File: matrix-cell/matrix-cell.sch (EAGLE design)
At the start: 4 parts

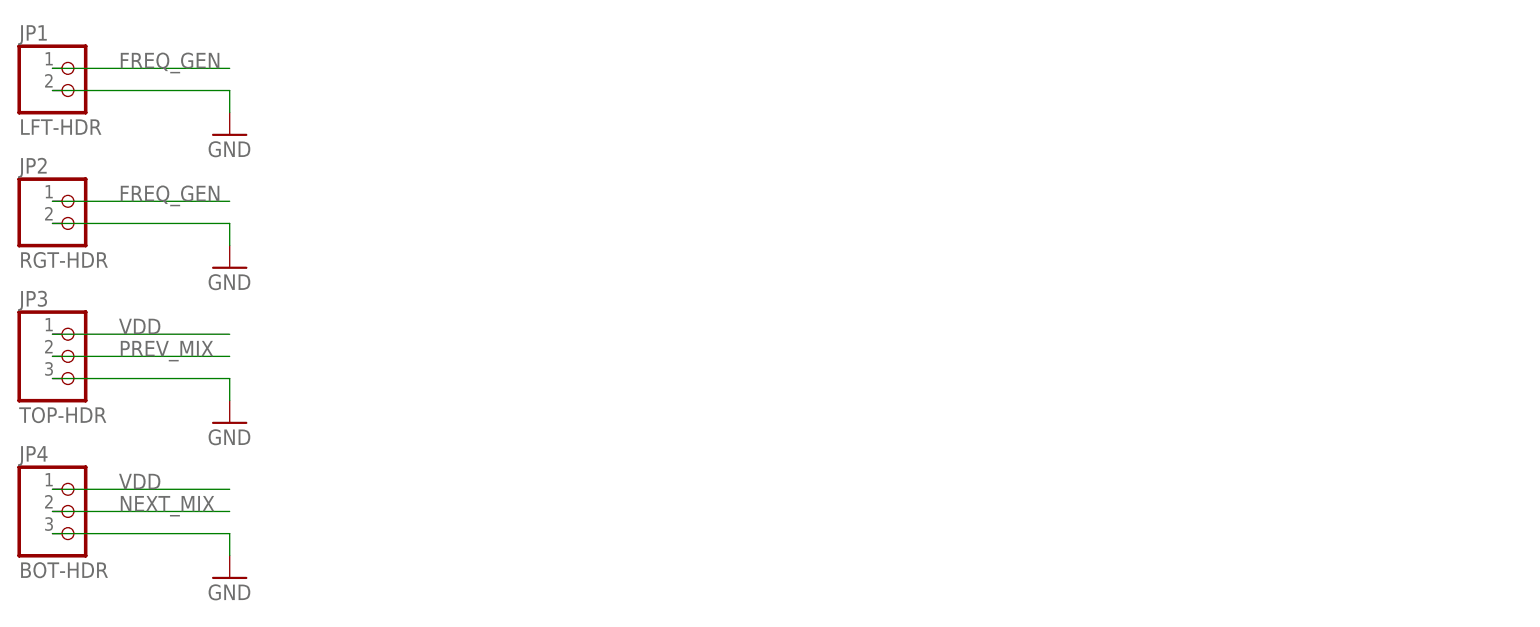
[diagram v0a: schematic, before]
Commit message: finished cell
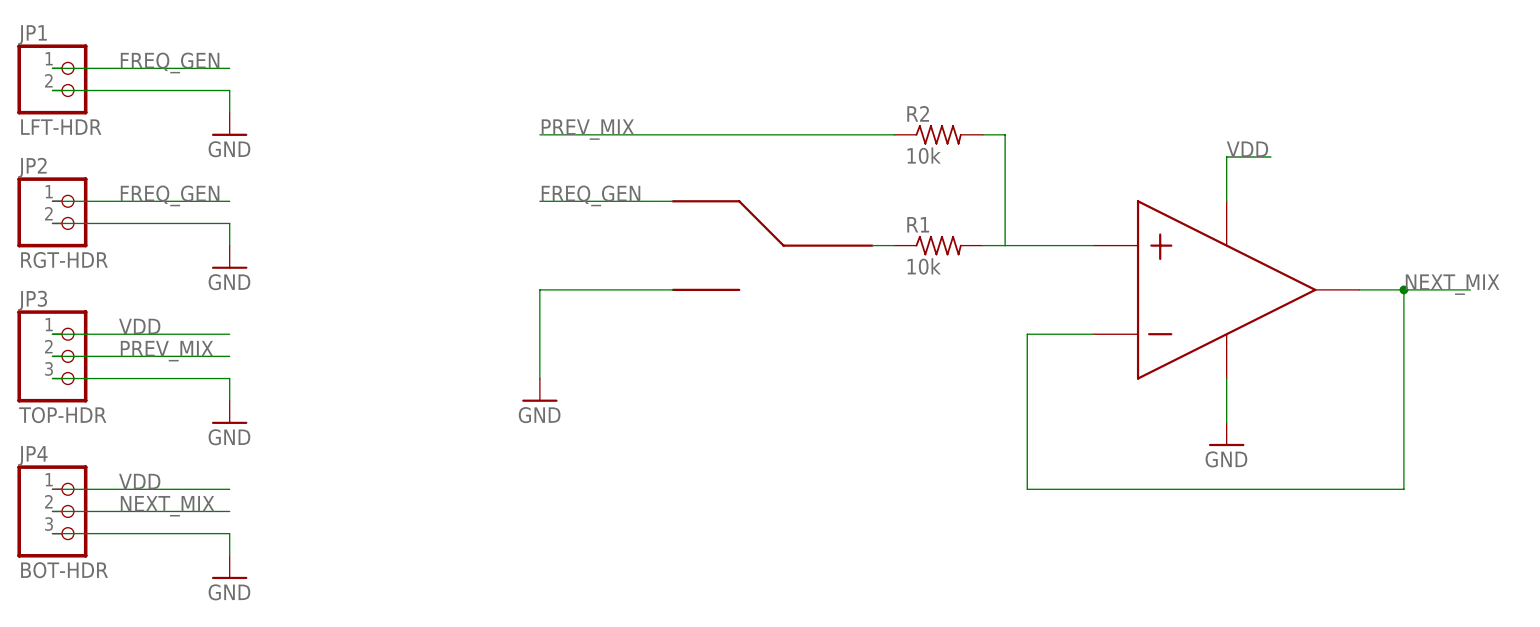
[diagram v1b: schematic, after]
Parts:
- added R1, R2: 10k, rcl:R-US_R1206
- added U$1: RA1-SWITCH, Tone-Matrix:RA1-SWITCH
- added U$2: MCP4162-OPAMP, Tone-Matrix:MCP4162-OPAMP
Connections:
- new net N$1: R1.2, R2.2, U$2.NON-INV
- new net N$2: R1.1, U$1.COMM
- net FREQ_GEN: now also U$1.NO
- net GND: now also U$1.NC, U$2.VSS
- net NEXT_MIX: now also U$2.INV, U$2.OUT
- net PREV_MIX: now also R2.1
- net VDD: now also U$2.VDD
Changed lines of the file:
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@@
 <part name="GND3" library="supply1" deviceset="GND" device=""/>
 <part name="GND4" library="supply1" deviceset="GND" device=""/>
+<part name="U$1" library="Tone-Matrix" deviceset="RA1-SWITCH" device=""/>
+<part name="U$2" library="Tone-Matrix" deviceset="MCP4162-OPAMP" device=""/>
+<part name="GND5" library="supply1" deviceset="GND" device=""/>
+<part name="R1" library="rcl" deviceset="R-US_" device="R1206" value="10k"/>
+<part name="R2" library="rcl" deviceset="R-US_" device="R1206" value="10k"/>
+<part name="GND6" library="supply1" deviceset="GND" device=""/>
 </parts>
 <sheets>
@@
 <instance part="GND3" gate="1" x="48.26" y="30.48"/>
 <instance part="GND4" gate="1" x="48.26" y="45.72"/>
+<instance part="U$1" gate="G$1" x="111.76" y="33.02" rot="MR0"/>
+<instance part="U$2" gate="G$1" x="152.4" y="20.32"/>
+<instance part="GND5" gate="1" x="162.56" y="10.16"/>
+<instance part="R1" gate="G$1" x="129.54" y="33.02"/>
+<instance part="R2" gate="G$1" x="129.54" y="45.72"/>
+<instance part="GND6" gate="1" x="83.82" y="15.24"/>
 </instances>
 <busses>
@@
 <label x="35.56" y="38.1" size="1.778" layer="95"/>
 </segment>
+<segment>
+<pinref part="U$1" gate="G$1" pin="NO"/>
+<wire x1="99.06" y1="38.1" x2="83.82" y2="38.1" width="0.1524" layer="91"/>
+<label x="83.82" y="38.1" size="1.778" layer="95"/>
+</segment>
 </net>
 <net name="VDD" class="0">
@@
 <label x="35.56" y="5.08" size="1.778" layer="95"/>
 </segment>
+<segment>
+<pinref part="U$2" gate="G$1" pin="VDD"/>
+<wire x1="162.56" y1="38.1" x2="162.56" y2="43.18" width="0.1524" layer="91"/>
+<wire x1="162.56" y1="43.18" x2="167.64" y2="43.18" width="0.1524" layer="91"/>
+<label x="162.56" y="43.18" size="1.778" layer="95"/>
+</segment>
 </net>
 <net name="PREV_MIX" class="0">
@@
 <label x="35.56" y="20.32" size="1.778" layer="95"/>
 </segment>
+<segment>
+<pinref part="R2" gate="G$1" pin="1"/>
+<wire x1="124.46" y1="45.72" x2="83.82" y2="45.72" width="0.1524" layer="91"/>
+<label x="83.82" y="45.72" size="1.778" layer="95"/>
+</segment>
 </net>
 <net name="NEXT_MIX" class="0">
@@
 <wire x1="27.94" y1="2.54" x2="48.26" y2="2.54" width="0.1524" layer="91"/>
 <label x="35.56" y="2.54" size="1.778" layer="95"/>
+</segment>
+<segment>
+<pinref part="U$2" gate="G$1" pin="INV"/>
+<wire x1="147.32" y1="22.86" x2="139.7" y2="22.86" width="0.1524" layer="91"/>
+<wire x1="139.7" y1="22.86" x2="139.7" y2="5.08" width="0.1524" layer="91"/>
+<wire x1="139.7" y1="5.08" x2="182.88" y2="5.08" width="0.1524" layer="91"/>
+<wire x1="182.88" y1="5.08" x2="182.88" y2="27.94" width="0.1524" layer="91"/>
+<pinref part="U$2" gate="G$1" pin="OUT"/>
+<wire x1="182.88" y1="27.94" x2="177.8" y2="27.94" width="0.1524" layer="91"/>
+<wire x1="182.88" y1="27.94" x2="190.5" y2="27.94" width="0.1524" layer="91"/>
+<label x="182.88" y="27.94" size="1.778" layer="95"/>
+<junction x="182.88" y="27.94"/>
 </segment>
 </net>
@@
 <pinref part="GND4" gate="1" pin="GND"/>
 </segment>
+<segment>
+<pinref part="U$2" gate="G$1" pin="VSS"/>
+<wire x1="162.56" y1="17.78" x2="162.56" y2="12.7" width="0.1524" layer="91"/>
+<pinref part="GND5" gate="1" pin="GND"/>
+</segment>
+<segment>
+<pinref part="U$1" gate="G$1" pin="NC"/>
+<wire x1="99.06" y1="27.94" x2="83.82" y2="27.94" width="0.1524" layer="91"/>
+<wire x1="83.82" y1="27.94" x2="83.82" y2="17.78" width="0.1524" layer="91"/>
+<pinref part="GND6" gate="1" pin="GND"/>
+</segment>
 </net>
+<net name="N$1" class="0">
+<segment>
+<pinref part="U$2" gate="G$1" pin="NON-INV"/>
+<pinref part="R1" gate="G$1" pin="2"/>
+<wire x1="147.32" y1="33.02" x2="137.16" y2="33.02" width="0.1524" layer="91"/>
+<pinref part="R2" gate="G$1" pin="2"/>
+<wire x1="137.16" y1="33.02" x2="134.62" y2="33.02" width="0.1524" layer="91"/>
+<wire x1="134.62" y1="45.72" x2="137.16" y2="45.72" width="0.1524" layer="91"/>
+<wire x1="137.16" y1="45.72" x2="137.16" y2="33.02" width="0.1524" layer="91"/>
+</segment>
+</net>
+<net name="N$2" class="0">
+<segment>
+<pinref part="R1" gate="G$1" pin="1"/>
+<pinref part="U$1" gate="G$1" pin="COMM"/>
+<wire x1="124.46" y1="33.02" x2="121.92" y2="33.02" width="0.1524" layer="91"/>
+</segment>
+</net>
